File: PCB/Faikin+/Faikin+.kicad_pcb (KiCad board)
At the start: 2 copper layers, 70 x 70 mm, 32 parts, among them J1 1x5, J2 Shelly, J3 USB-PROG, J4 1x5, Q1 BSS138PS, Q2 BSS138PS, U3 MD8942, U4 ESP32-S3-MINI-1

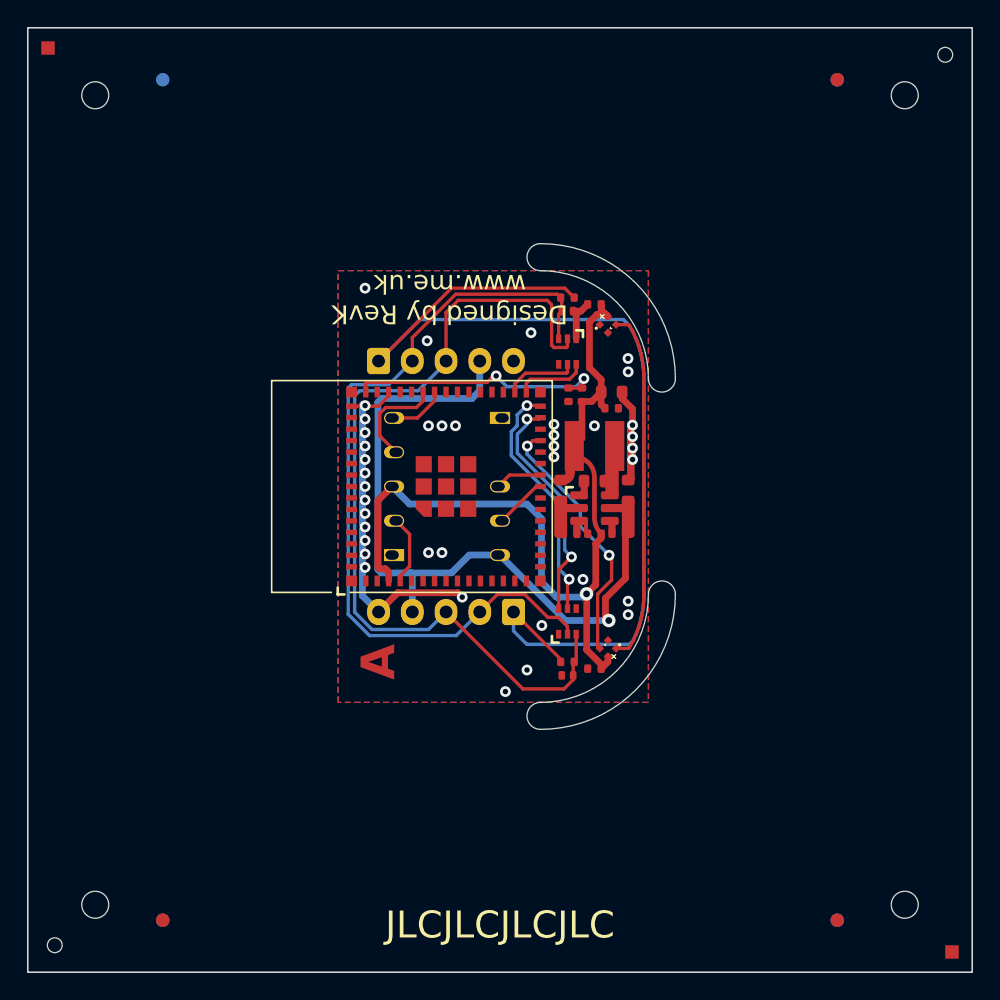
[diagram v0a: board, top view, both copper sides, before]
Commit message: New header
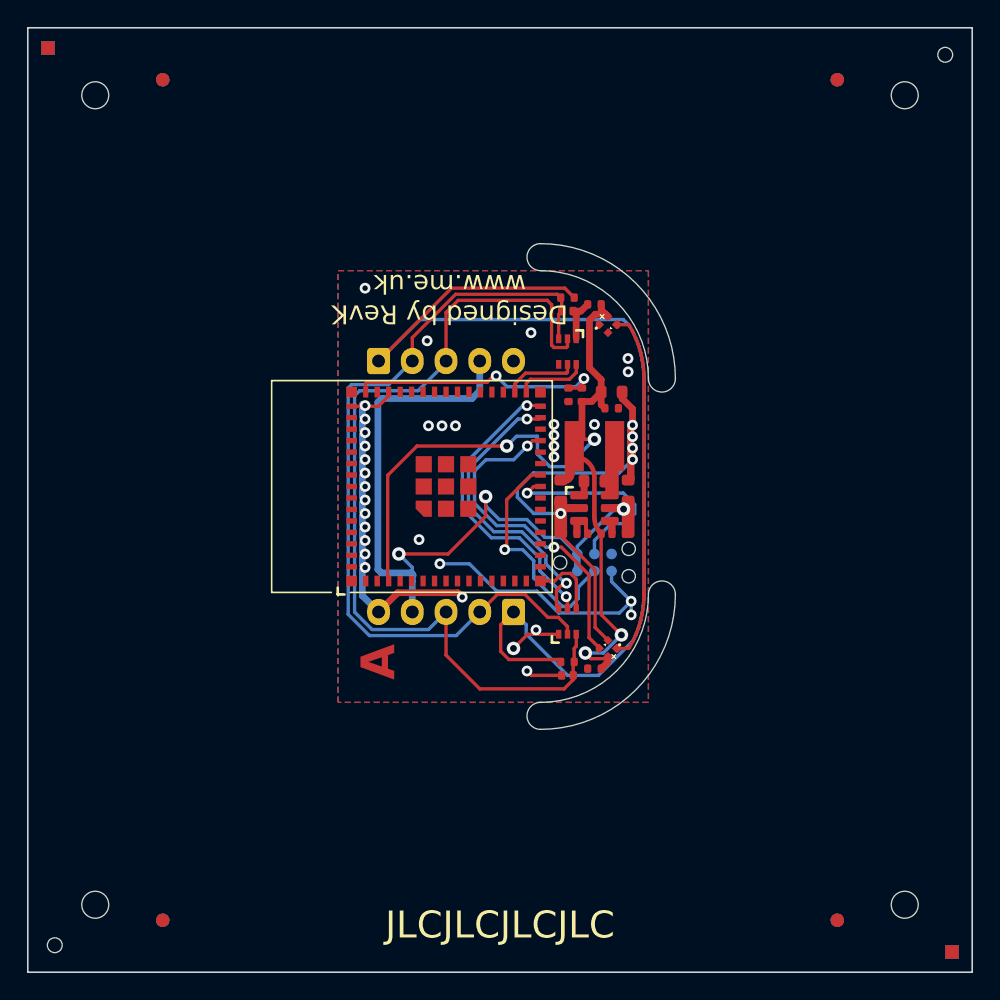
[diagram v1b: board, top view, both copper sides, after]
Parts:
- removed J2: Shelly, RevK:Shelly
- removed J3: USB-PROG, RevK:USB-PROG
- added J5: TC2030-USB-NL-DS, RevK:Tag-Connect_TC2030-IDC-NL_2x03_P1.27mm_Vertical, B.Cu at (142.0, 69.6)
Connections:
- U4 pad 39: Net-(J2-Tx) -> unconnected-(U4-GPIO43-Pad39)
- U4 pad 4: Net-(J2-0) -> unconnected-(U4-GPIO0-Pad4)
- U4 pad 40: Net-(J2-Rx) -> unconnected-(U4-GPIO44-Pad40)
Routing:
- net GND: track 36.2 -> 91.1 mm
- net D+: track 3.50 -> 17.8 mm, vias 0 -> 1
- net D-: track 3.90 -> 15.0 mm, vias 0 -> 1
- net Net-(J2-Rx): track 7.64 -> 0.00 mm
- net LED: track 19.2 -> 24.7 mm
- net Net-(J2-0): track 5.16 -> 0.00 mm
- net RX: track 17.4 -> 22.1 mm
- net Net-(J1-Pin_1): track 76.7 -> 81.1 mm
- net Net-(J2-Tx): track 4.33 -> 0.00 mm
- net TX: track 18.3 -> 22.6 mm
- net DC: track 52.2 -> 55.1 mm, vias 1 -> 3
- net S21TX: track 63.9 -> 65.8 mm
- net +3.3V: track 55.6 -> 57.2 mm, vias 1 -> 4

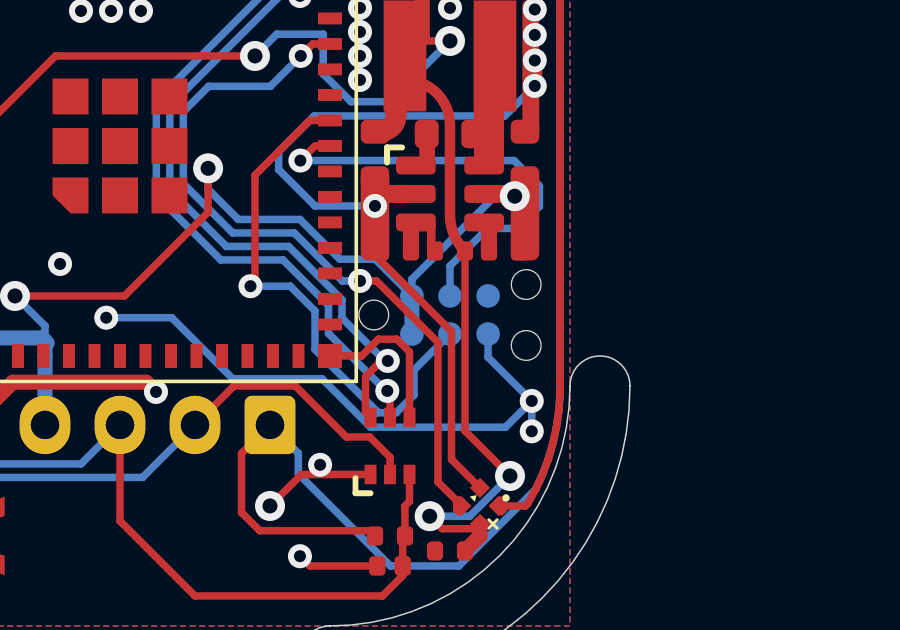
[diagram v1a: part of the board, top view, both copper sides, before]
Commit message: Style
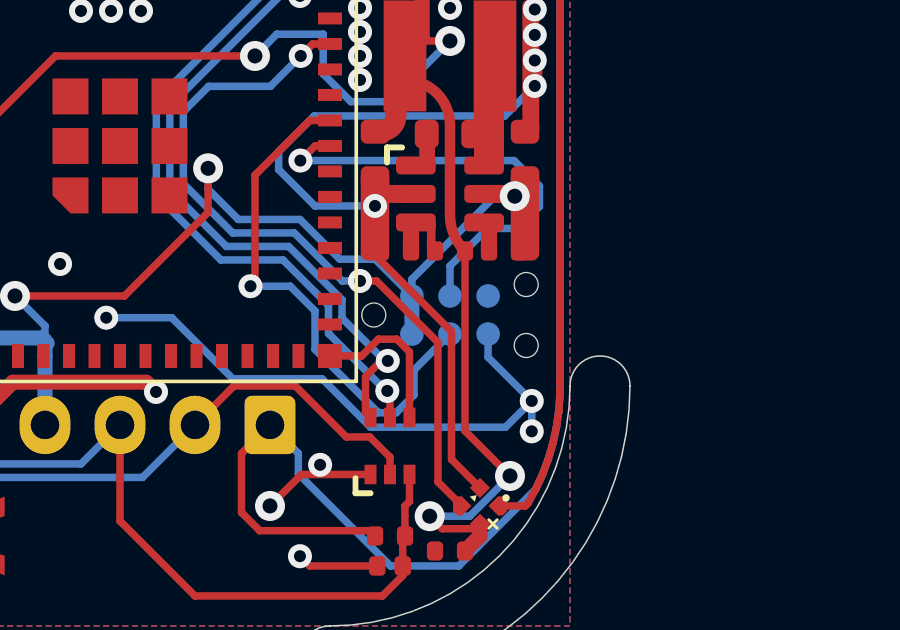
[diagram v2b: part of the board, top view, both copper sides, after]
